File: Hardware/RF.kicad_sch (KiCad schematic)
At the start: 0 parts

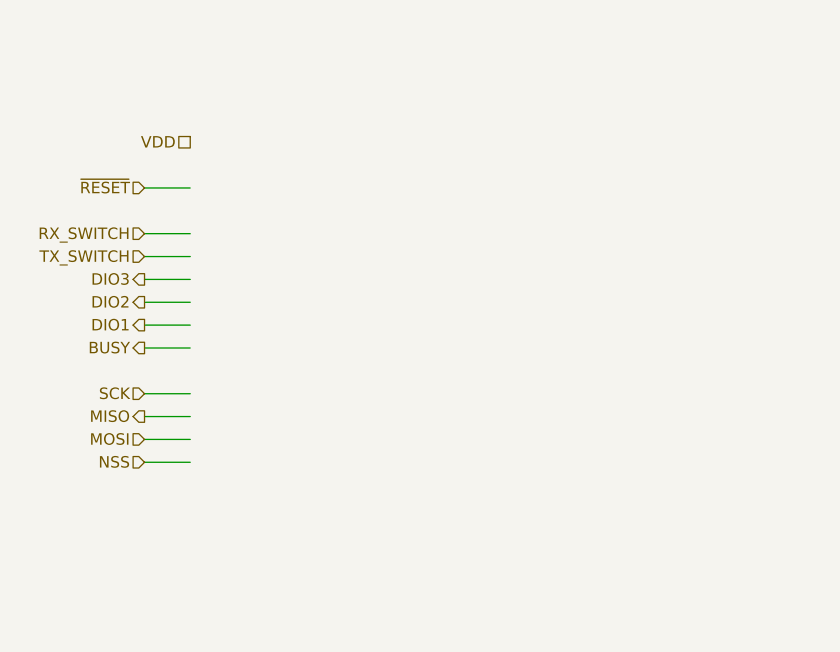
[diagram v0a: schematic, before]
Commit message: Checkpoint
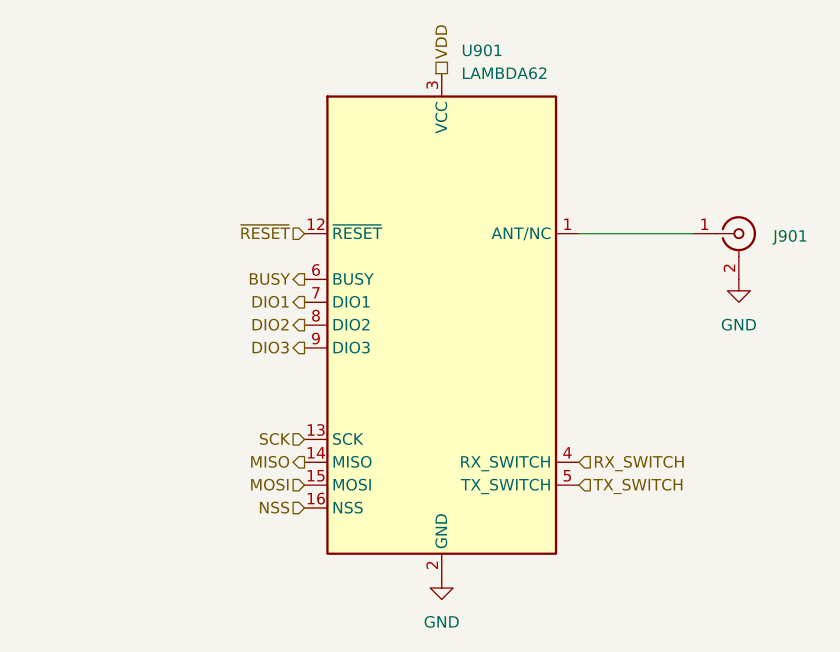
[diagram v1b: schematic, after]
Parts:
- added J901: ~, Connector_Coaxial:SMA_Amphenol_132134_Vertical, symbol Connector:Conn_Coaxial
- added U901: LAMBDA62, leptunKicadLib:LAMBDA62, symbol leptunKicadLib:LAMBDA62
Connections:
- net BUSY: now also U901.6 (BUSY)
- net DIO1: now also U901.7 (DIO1)
- net DIO2: now also U901.8 (DIO2)
- net DIO3: now also U901.9 (DIO3)
- net MISO: now also U901.14 (MISO)
- net MOSI: now also U901.15 (MOSI)
- net NSS: now also U901.16 (NSS)
- net RX_SWITCH: now also U901.4 (RX_SWITCH)
- net SCK: now also U901.13 (SCK)
- net TX_SWITCH: now also U901.5 (TX_SWITCH)
- net VDD: now also U901.3 (VCC)
- net ~{RESET}: now also U901.12 (~{RESET})
- new net: J901.1 (In), U901.1 (ANT/NC)
- new net GND: J901.2 (Ext), U901.2 (GND)
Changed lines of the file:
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@@
 (kicad_sch (version 20230121) (generator eeschema)
   (paper "A4")
-  (wire (pts (xy 114.3 86.36) (xy 119.38 86.36))
+  (wire (pts (xy 162.56 83.82) (xy 175.26 83.82))
     (stroke (width 0) (type default))
   )
-  (wire (pts (xy 114.3 78.74) (xy 119.38 78.74))
-    (stroke (width 0) (type default))
+  (hierarchical_label "TX_SWITCH" (shape input) (at 162.56 111.76 0) (fields_autoplaced)
+    (effects (font (size 1.27 1.27)) (justify left))
   )
-  (wire (pts (xy 114.3 96.52) (xy 119.38 96.52))
-    (stroke (width 0) (type default))
+  (hierarchical_label "RX_SWITCH" (shape input) (at 162.56 109.22 0) (fields_autoplaced)
+    (effects (font (size 1.27 1.27)) (justify left))
   )
-  (wire (pts (xy 114.3 91.44) (xy 119.38 91.44))
-    (stroke (width 0) (type default))
-  )
-  (wire (pts (xy 114.3 88.9) (xy 119.38 88.9))
-    (stroke (width 0) (type default))
-  )
-  (wire (pts (xy 114.3 101.6) (xy 119.38 101.6))
-    (stroke (width 0) (type default))
-  )
-  (wire (pts (xy 114.3 93.98) (xy 119.38 93.98))
-    (stroke (width 0) (type default))
-  )
-  (wire (pts (xy 114.3 109.22) (xy 119.38 109.22))
-    (stroke (width 0) (type default))
-  )
-  (wire (pts (xy 114.3 104.14) (xy 119.38 104.14))
-    (stroke (width 0) (type default))
-  )
-  (wire (pts (xy 114.3 106.68) (xy 119.38 106.68))
-    (stroke (width 0) (type default))
-  )
-  (wire (pts (xy 114.3 83.82) (xy 119.38 83.82))
-    (stroke (width 0) (type default))
-  )
-  (hierarchical_label "TX_SWITCH" (shape input) (at 114.3 86.36 180) (fields_autoplaced)
+  (hierarchical_label "MOSI" (shape input) (at 132.08 111.76 180) (fields_autoplaced)
     (effects (font (size 1.27 1.27)) (justify right))
   )
-  (hierarchical_label "RX_SWITCH" (shape input) (at 114.3 83.82 180) (fields_autoplaced)
+  (hierarchical_label "NSS" (shape input) (at 132.08 114.3 180) (fields_autoplaced)
     (effects (font (size 1.27 1.27)) (justify right))
   )
-  (hierarchical_label "MOSI" (shape input) (at 114.3 106.68 180) (fields_autoplaced)
+  (hierarchical_label "~{RESET}" (shape input) (at 132.08 83.82 180) (fields_autoplaced)
     (effects (font (size 1.27 1.27)) (justify right))
   )
-  (hierarchical_label "NSS" (shape input) (at 114.3 109.22 180) (fields_autoplaced)
+  (hierarchical_label "MISO" (shape output) (at 132.08 109.22 180) (fields_autoplaced)
     (effects (font (size 1.27 1.27)) (justify right))
   )
-  (hierarchical_label "~{RESET}" (shape input) (at 114.3 78.74 180) (fields_autoplaced)
+  (hierarchical_label "DIO2" (shape output) (at 132.08 93.98 180) (fields_autoplaced)
     (effects (font (size 1.27 1.27)) (justify right))
   )
-  (hierarchical_label "MISO" (shape output) (at 114.3 104.14 180) (fields_autoplaced)
+  (hierarchical_label "VDD" (shape passive) (at 147.32 66.04 90) (fields_autoplaced)
+    (effects (font (size 1.27 1.27)) (justify left))
+  )
+  (hierarchical_label "SCK" (shape input) (at 132.08 106.68 180) (fields_autoplaced)
     (effects (font (size 1.27 1.27)) (justify right))
   )
-  (hierarchical_label "DIO2" (shape output) (at 114.3 91.44 180) (fields_autoplaced)
+  (hierarchical_label "DIO1" (shape output) (at 132.08 91.44 180) (fields_autoplaced)
     (effects (font (size 1.27 1.27)) (justify right))
   )
-  (hierarchical_label "VDD" (shape passive) (at 119.38 73.66 180) (fields_autoplaced)
+  (hierarchical_label "DIO3" (shape output) (at 132.08 96.52 180) (fields_autoplaced)
     (effects (font (size 1.27 1.27)) (justify right))
   )
-  (hierarchical_label "SCK" (shape input) (at 114.3 101.6 180) (fields_autoplaced)
+  (hierarchical_label "BUSY" (shape output) (at 132.08 88.9 180) (fields_autoplaced)
     (effects (font (size 1.27 1.27)) (justify right))
   )
-  (hierarchical_label "DIO1" (shape output) (at 114.3 93.98 180) (fields_autoplaced)
-    (effects (font (size 1.27 1.27)) (justify right))
+  (symbol (lib_id "power:GND") (at 180.34 88.9 0) (unit 1)
+    (in_bom yes) (on_board yes) (dnp no) (fields_autoplaced)
+    (property "Reference" "#PWR0902" (at 180.34 95.25 0)
+      (effects (font (size 1.27 1.27)) hide)
+    )
+    (property "Value" "GND" (at 180.34 93.98 0)
+      (effects (font (size 1.27 1.27)))
+    )
+    (property "Footprint" "" (at 180.34 88.9 0)
+      (effects (font (size 1.27 1.27)) hide)
+    )
+    (property "Datasheet" "" (at 180.34 88.9 0)
+      (effects (font (size 1.27 1.27)) hide)
+    )
+    (pin "1")
+    (instances
+      (project "Avionus_Flight_Controller"
+        (path "/ddc7e940-0588-4587-8902-8ced9e615ace/a9aaa4a3-7ef9-4aeb-9917-54b44867eb01"
+          (reference "#PWR0902") (unit 1)
+        )
+      )
+    )
   )
-  (hierarchical_label "DIO3" (shape output) (at 114.3 88.9 180) (fields_autoplaced)
-    (effects (font (size 1.27 1.27)) (justify right))
+  (symbol (lib_id "Connector:Conn_Coaxial") (at 180.34 83.82 0) (unit 1)
+    (in_bom yes) (on_board yes) (dnp no) (fields_autoplaced)
+    (property "Reference" "J901" (at 184.15 84.1132 0)
+      (effects (font (size 1.27 1.27)) (justify left))
+    )
+    (property "Value" "~" (at 184.15 85.3832 0)
+      (effects (font (size 1.27 1.27)) (justify left))
+    )
+    (property "Footprint" "Connector_Coaxial:SMA_Amphenol_132134_Vertical" (at 180.34 83.82 0)
+      (effects (font (size 1.27 1.27)) hide)
+    )
+    (property "Datasheet" " ~" (at 180.34 83.82 0)
+      (effects (font (size 1.27 1.27)) hide)
+    )
+    (pin "1")
+    (pin "2")
+    (instances
+      (project "Avionus_Flight_Controller"
+        (path "/ddc7e940-0588-4587-8902-8ced9e615ace/a9aaa4a3-7ef9-4aeb-9917-54b44867eb01"
+          (reference "J901") (unit 1)
+        )
+      )
+    )
   )
-  (hierarchical_label "BUSY" (shape output) (at 114.3 96.52 180) (fields_autoplaced)
-    (effects (font (size 1.27 1.27)) (justify right))
+  (symbol (lib_id "leptunKicadLib:LAMBDA62") (at 147.32 93.98 0) (unit 1)
+    (in_bom yes) (on_board yes) (dnp no) (fields_autoplaced)
+    (property "Reference" "U901" (at 149.5141 63.5 0)
+      (effects (font (size 1.27 1.27)) (justify left))
+    )
+    (property "Value" "LAMBDA62" (at 149.5141 66.04 0)
+      (effects (font (size 1.27 1.27)) (justify left))
+    )
+    (property "Footprint" "leptunKicadLib:LAMBDA62" (at 147.32 101.6 0)
+      (effects (font (size 1.27 1.27)) hide)
+    )
+    (property "Datasheet" "https://www.rfsolutions.co.uk/downloads/63c81a2964da3203DS-LAMBDA62-6.pdf" (at 147.32 99.06 0)
+      (effects (font (size 1.27 1.27)) hide)
+    )
+    (pin "1")
+    (pin "10")
+    (pin "11")
+    (pin "12")
+    (pin "13")
+    (pin "14")
+    (pin "15")
+    (pin "16")
+    (pin "2")
+    (pin "3")
+    (pin "4")
+    (pin "5")
+    (pin "6")
+    (pin "7")
+    (pin "8")
+    (pin "9")
+    (instances
+      (project "Avionus_Flight_Controller"
+        (path "/ddc7e940-0588-4587-8902-8ced9e615ace/a9aaa4a3-7ef9-4aeb-9917-54b44867eb01"
+          (reference "U901") (unit 1)
+        )
+      )
+    )
+  )
+  (symbol (lib_id "power:GND") (at 147.32 121.92 0) (unit 1)
+    (in_bom yes) (on_board yes) (dnp no) (fields_autoplaced)
+    (property "Reference" "#PWR0901" (at 147.32 128.27 0)
+      (effects (font (size 1.27 1.27)) hide)
+    )
+    (property "Value" "GND" (at 147.32 127 0)
+      (effects (font (size 1.27 1.27)))
+    )
+    (property "Footprint" "" (at 147.32 121.92 0)
+      (effects (font (size 1.27 1.27)) hide)
+    )
+    (property "Datasheet" "" (at 147.32 121.92 0)
+      (effects (font (size 1.27 1.27)) hide)
+    )
+    (pin "1")
+    (instances
+      (project "Avionus_Flight_Controller"
+        (path "/ddc7e940-0588-4587-8902-8ced9e615ace/a9aaa4a3-7ef9-4aeb-9917-54b44867eb01"
+          (reference "#PWR0901") (unit 1)
+        )
+      )
+    )
   )
 )
